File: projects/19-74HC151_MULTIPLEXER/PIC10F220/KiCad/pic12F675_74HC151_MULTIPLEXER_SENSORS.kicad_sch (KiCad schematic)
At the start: 10 parts, among them U1 PIC12F675-IP, U3 MQ-2

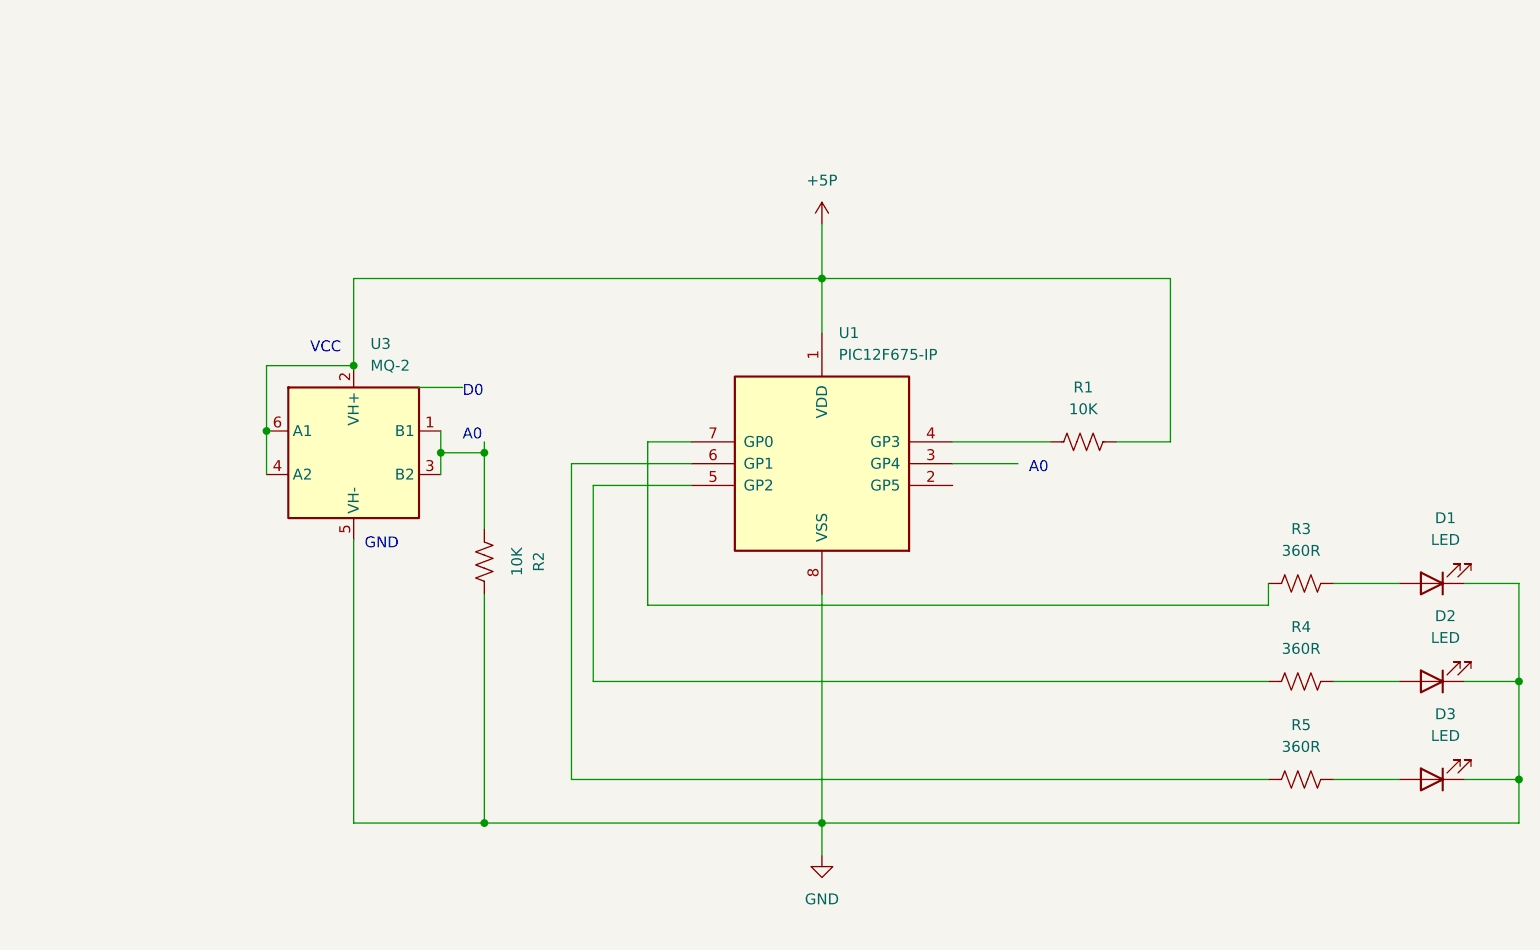
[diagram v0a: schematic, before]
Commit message: Doc
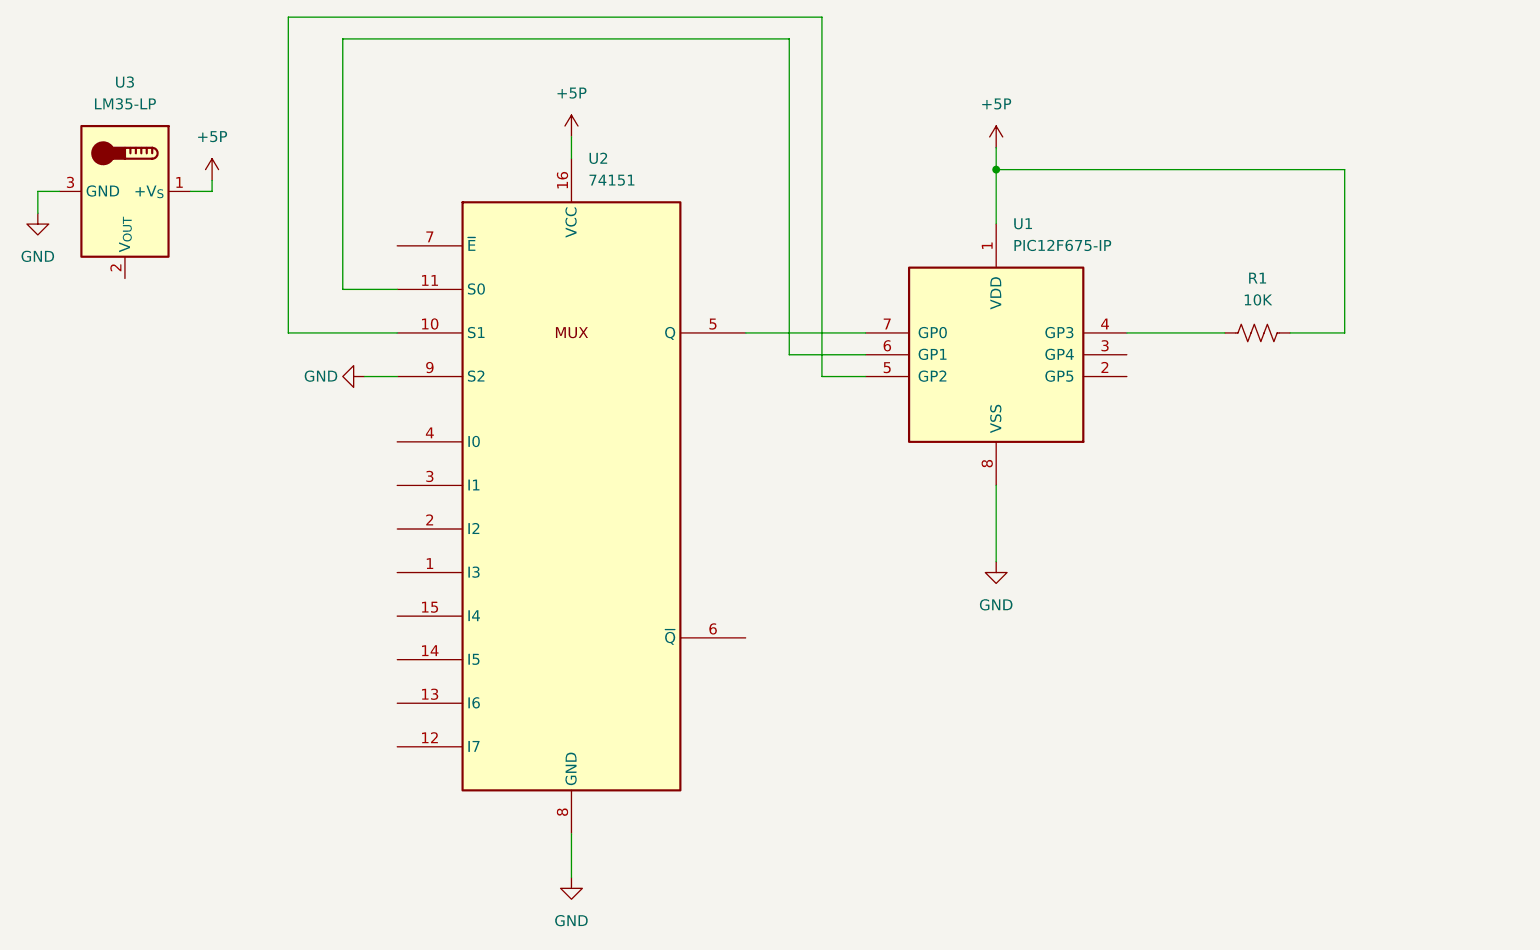
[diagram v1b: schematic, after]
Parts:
- removed D1, D2, D3: LED, symbol Device:LED
- removed R2: 10K, symbol Device:R_US
- removed R3, R4, R5: 360R, symbol Device:R_US
- removed U3: MQ-2, Sensor:MQ-6, symbol Sensor_Gas:MQ-6
- added U2: 74151, symbol 74xx_IEEE:74151
- added U3: LM35-LP, Package_TO_SOT_THT:TO-92_Inline, symbol Sensor_Temperature:LM35-LP
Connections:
- net +5P: now also U2.16 (VCC), U3.1 (+V_{S})
- net GND: now also U2.8 (GND), U2.9 (S2), U3.3 (GND)
- net at U1.7 (GP0): now also U2.5 (Q)
- net at U1.5 (GP2): now also U2.10 (S1)
- net at U1.6 (GP1): now also U2.11 (S0)
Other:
- note removed: "A0"
- note removed: "D0"
- note removed: "GND"
- note removed: "VCC"
- moved on the sheet: R1, U1
